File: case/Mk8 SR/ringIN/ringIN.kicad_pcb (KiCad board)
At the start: 2 copper layers, 30.9 x 30.9 mm, 0 parts

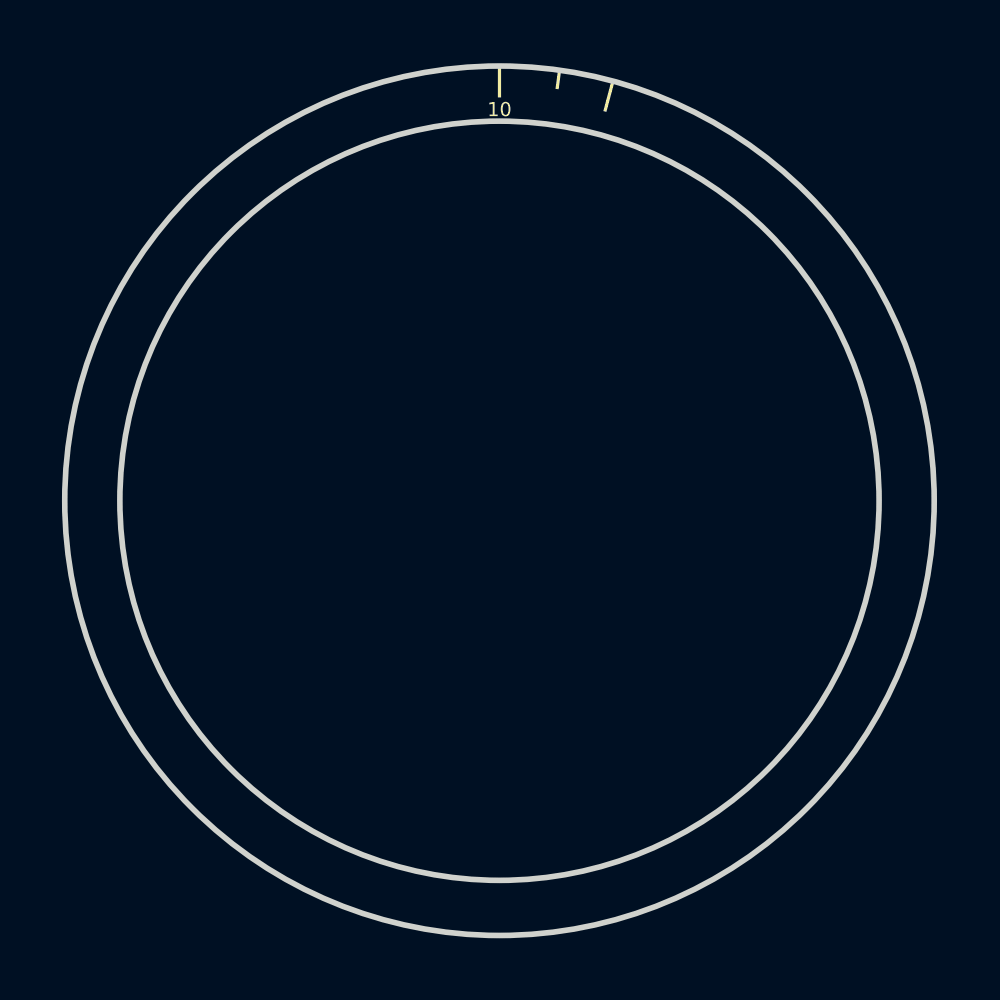
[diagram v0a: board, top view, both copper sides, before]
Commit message: working on new ring
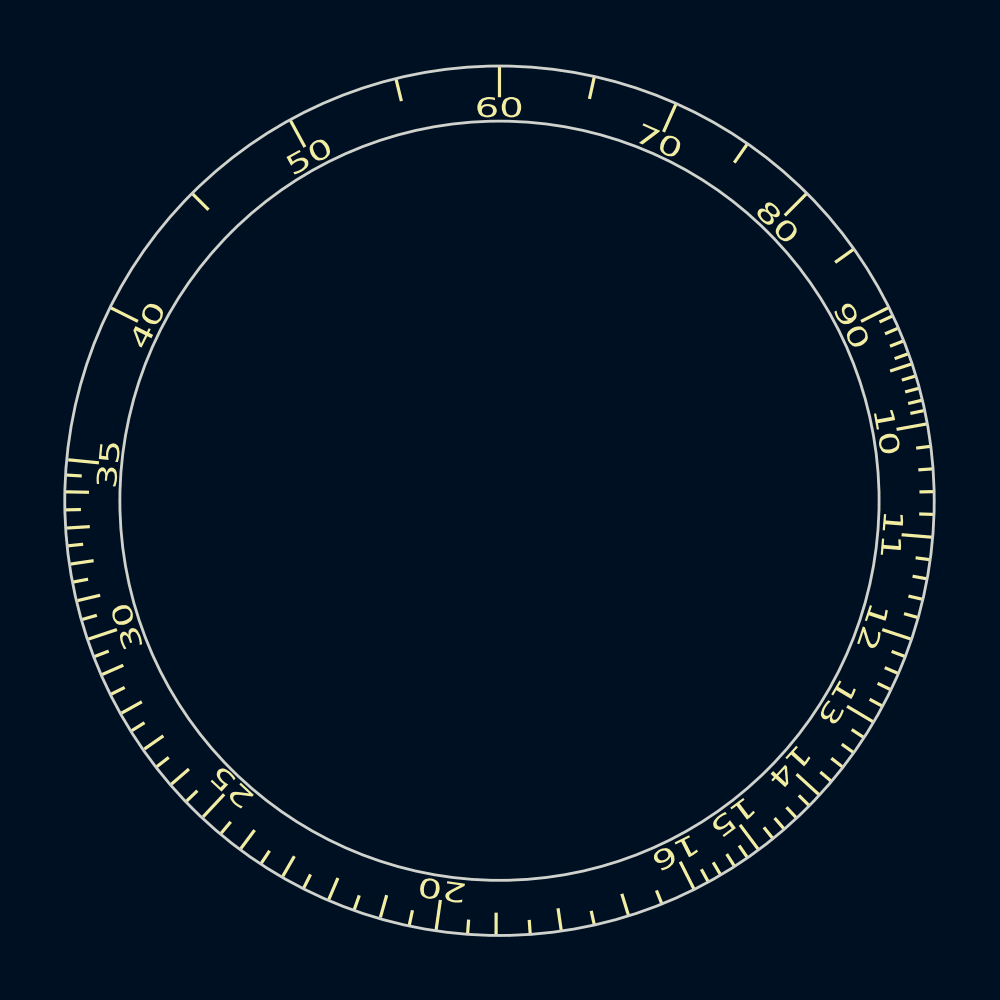
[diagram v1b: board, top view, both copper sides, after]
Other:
- board text added: "11"
- board text added: "12"
- board text added: "13"
- board text added: "14"
- board text added: "15"
- board text added: "16"
- board text added: "20"
- board text added: "25"
- board text added: "30"
- board text added: "35"
- board text added: "40"
- board text added: "50"
- board text added: "60"
- board text added: "70"
- board text added: "80"
- board text added: "90"
